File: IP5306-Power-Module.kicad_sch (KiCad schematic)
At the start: 25 parts, among them J1 USB_C_Receptacle_USB2.0_16P, J2 S2B-XH-A_LF__SN_, J3 USB_A, J4 USB_A, SW1 KEY, U1 IP5306

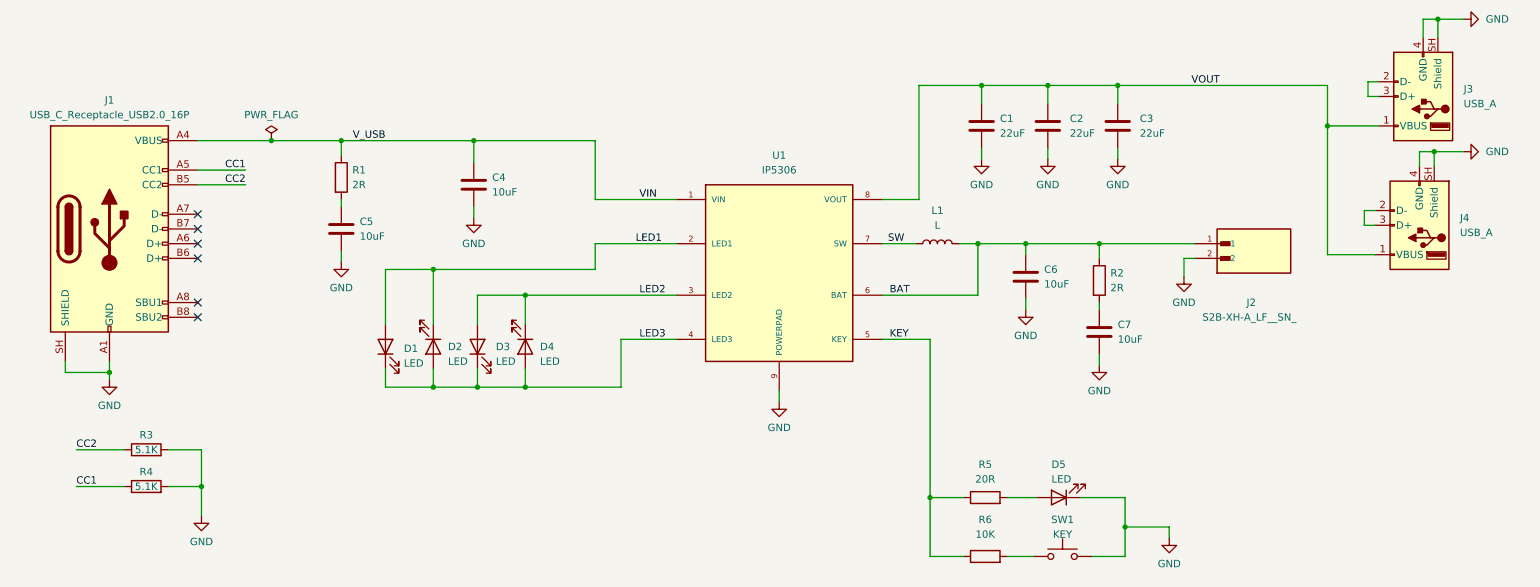
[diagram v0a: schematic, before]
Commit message: V1
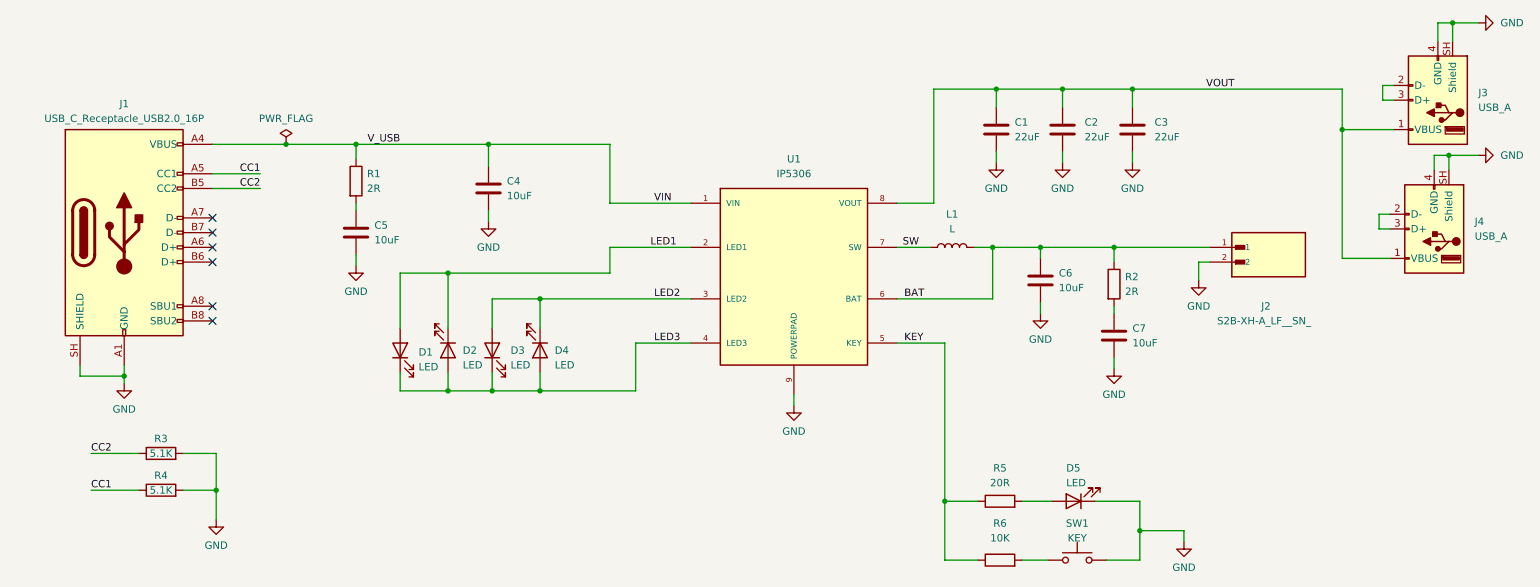
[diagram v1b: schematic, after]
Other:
- moved on the sheet: C1, C2, C3, C4, C5, C6, C7, D1, D2, D3, D4, D5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
